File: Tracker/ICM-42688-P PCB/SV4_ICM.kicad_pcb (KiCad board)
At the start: 2 copper layers, 17.8 x 26.5 mm, 21 parts, among them U1 SuperMini nRF52840, U2 ICM-42688-P, U3 MMC5983MA, U4 K3-1295S-E1

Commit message: - Changed speed for top layers in 3mf file - Added more pages to manual - Added 11-tracker dock
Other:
- board text added: "MP-S-4.4.2"
- board text removed: "MP-S-4.4.1"
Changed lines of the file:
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@@
 		)
 	)
-	(gr_text "MP-S-4.4.1"
+	(gr_text "MP-S-4.4.2"
 		(at 151.003 98.171 270)
 		(layer "B.Mask")

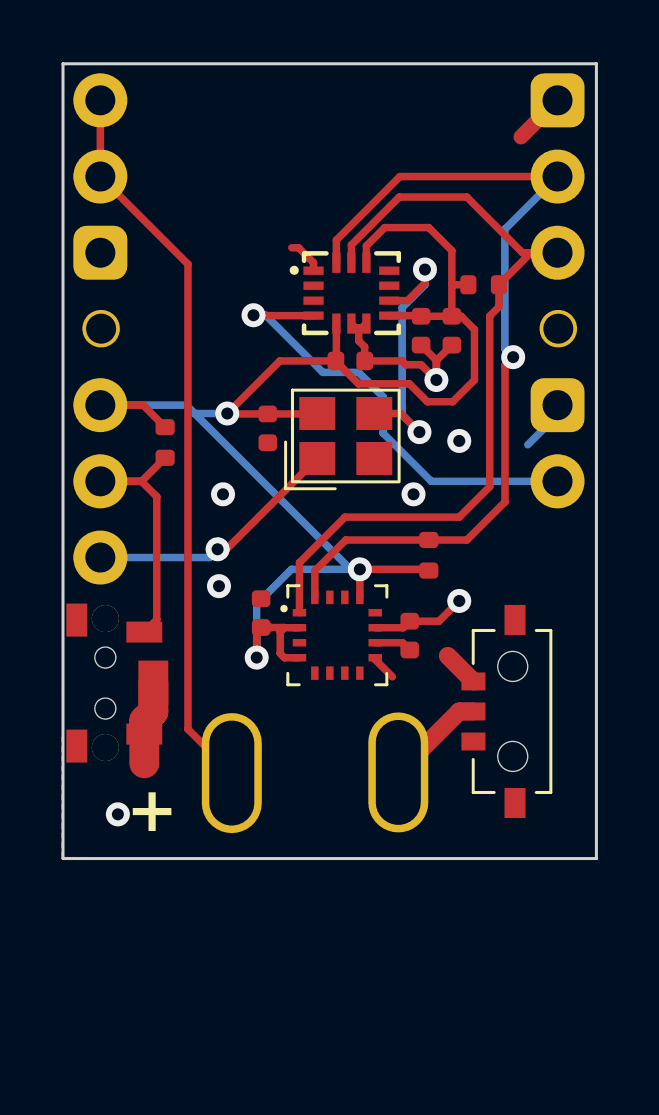
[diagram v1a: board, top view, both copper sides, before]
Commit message: - Started updating pcb for spi, didn't ifnish lol use the last commit - Added
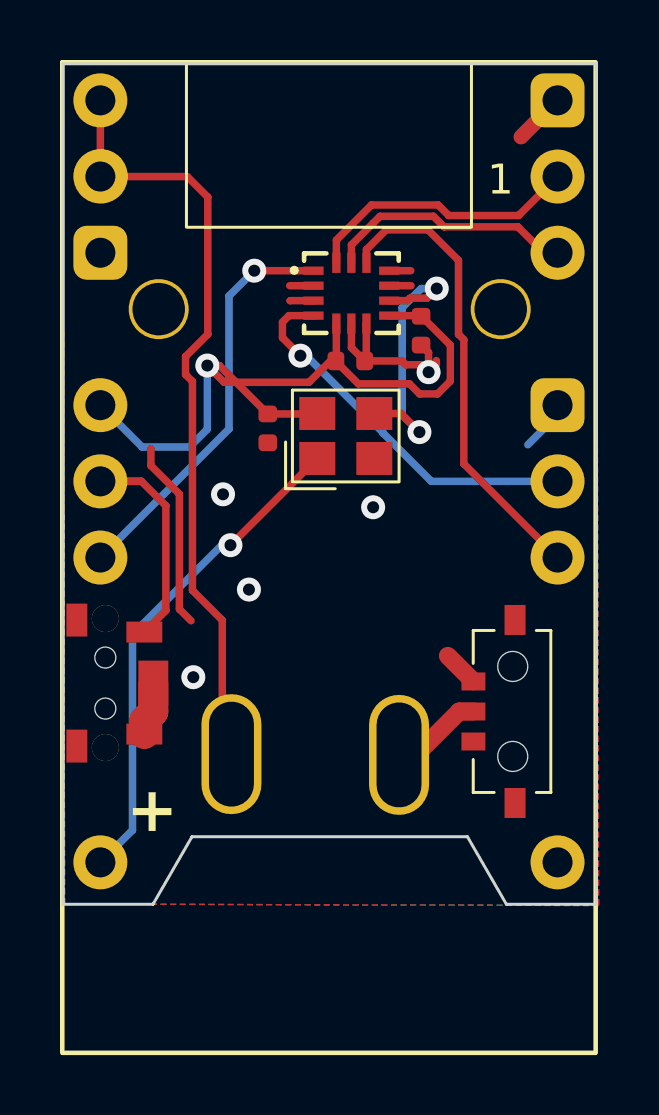
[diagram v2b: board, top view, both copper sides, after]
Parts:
- removed C2: 1uF, Capacitor_SMD:C_0402_1005Metric
- removed C5: 10uF, Capacitor_SMD:C_0402_1005Metric
- removed C7: 2.2uF, Capacitor_SMD:C_0402_1005Metric
- removed R1, R2: 10k, Resistor_SMD:R_0402_1005Metric
- removed R5: 200k, Resistor_SMD:R_0402_1005Metric
- removed U3: MMC5983MA, mag_custom:MMC5983MA
- C3: value 10nF -> 100nF
- moved REF** 2.04 mm to (138.1, 80.7)
- moved TP1 0.63 mm to (140.5, 95.5)
- moved TP2 0.58 mm to (146.1, 95.6)
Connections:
- net Net-(U2-INT2/FSYNC/CLKIN) renamed CLK
- REF** pad 1: (no net) -> GND
- U1 pad 18: OSC_EN -> SDO
- U2 pad 1: GND -> SDO
- U2 pad 12: +3V3 -> CS
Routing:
- net +3V3: track 53.9 -> 25.5 mm, vias 3 -> 1
- net SDA: track 29.0 -> 9.30 mm, vias 1 -> 0
- net SCL: track 27.2 -> 8.36 mm
- net CS: track 0.00 -> 15.5 mm
- net SDO: track 0.00 -> 13.7 mm, vias 0 -> 1
- net OSC_EN: track 8.60 -> 16.6 mm
- net INT1: track 15.6 -> 13.3 mm
- net Net-(TP1-Pad1): track 24.2 -> 26.5 mm
- net Net-(U3-CAP): track 1.25 -> 0.00 mm
- net GND: track 20.2 -> 19.3 mm, vias 7 -> 5
- net Net-(U1-P0.31-LF): track 9.26 -> 8.40 mm
- net unconnected-(U2-RESV-Pad2): track 0.00 -> 0.79 mm
- net unconnected-(U2-RESV-Pad3): track 0.00 -> 0.78 mm
- net unconnected-(U2-RESV-Pad10): track 0.00 -> 0.73 mm
- net unconnected-(U2-RESV-Pad11): track 0.00 -> 0.72 mm
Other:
- board size 17.8 x 26.5 mm -> 17.8 x 28 mm
